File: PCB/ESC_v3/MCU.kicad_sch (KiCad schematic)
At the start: 44 parts, among them J10 Conn_01x01_Pin, J3 Conn_01x01_Pin, J4 Conn_01x01_Pin, J5 Conn_01x01_Pin, J6 Conn_01x01_Pin, J7 Conn_01x01_Pin, J8 Conn_01x01_Pin, J9 Conn_01x01_Pin, U3 STM32G474CETx, Y2 24MHz

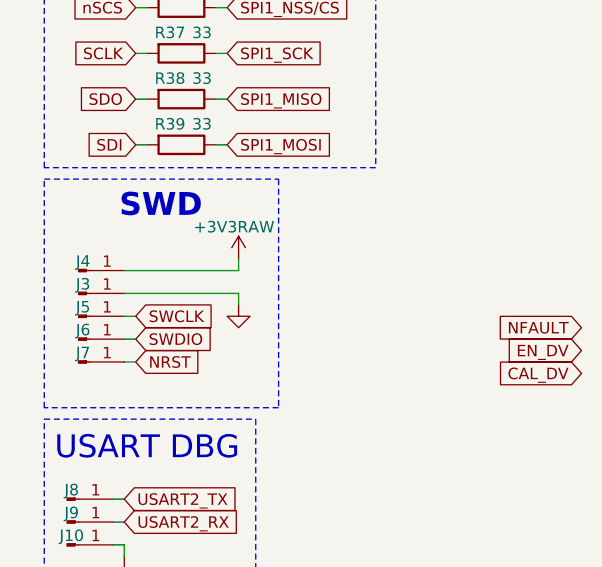
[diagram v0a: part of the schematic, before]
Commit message: Layout update
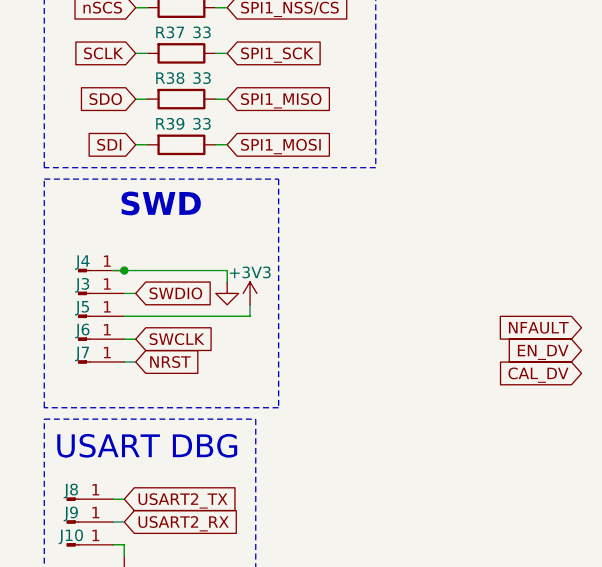
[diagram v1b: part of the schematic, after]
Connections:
- net +3V3RAW is gone; now on net GND: J4.1 (Pin_1)
- net +3V3: now also J5.1 (Pin_1)
- net GND: no longer J3.1 (Pin_1)
- net SWCLK: now also J6.1 (Pin_1); no longer J5.1 (Pin_1)
- net SWDIO: now also J3.1 (Pin_1); no longer J6.1 (Pin_1)
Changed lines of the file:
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@@
 	)
 	(junction
+		(at 25.4 109.22)
+		(diameter 0)
+		(color 0 0 0 0)
+	)
+	(junction
 		(at 43.18 179.07)
 		(diameter 0)
@@
 	(wire
 		(pts
-			(xy 25.4 109.22) (xy 38.1 109.22)
-		)
-		(stroke
-			(width 0)
-			(type default)
-		)
-	)
-	(wire
-		(pts
 			(xy 35.56 60.96) (xy 35.56 62.23)
 		)
@@
 	(wire
 		(pts
-			(xy 25.4 111.76) (xy 38.1 111.76)
-		)
-		(stroke
-			(width 0)
-			(type default)
-		)
-	)
-	(wire
-		(pts
 			(xy 139.7 67.31) (xy 137.16 67.31)
 		)
@@
 	(wire
 		(pts
+			(xy 26.67 111.76) (xy 25.4 111.76)
+		)
+		(stroke
+			(width 0)
+			(type default)
+		)
+	)
+	(wire
+		(pts
 			(xy 25.4 137.16) (xy 24.13 137.16)
 		)
@@
 	(wire
 		(pts
-			(xy 38.1 107.95) (xy 38.1 109.22)
+			(xy 39.37 113.03) (xy 39.37 114.3)
 		)
 		(stroke
@@
 	(wire
 		(pts
-			(xy 38.1 111.76) (xy 38.1 113.03)
+			(xy 36.83 109.22) (xy 36.83 110.49)
 		)
 		(stroke
@@
 	(wire
 		(pts
+			(xy 24.13 109.22) (xy 25.4 109.22)
+		)
+		(stroke
+			(width 0)
+			(type default)
+		)
+	)
+	(wire
+		(pts
 			(xy 43.18 187.96) (xy 43.18 189.23)
 		)
@@
 	(wire
 		(pts
+			(xy 25.4 109.22) (xy 36.83 109.22)
+		)
+		(stroke
+			(width 0)
+			(type default)
+		)
+	)
+	(wire
+		(pts
 			(xy 35.56 85.09) (xy 36.83 85.09)
 		)
@@
 	(wire
 		(pts
-			(xy 26.67 114.3) (xy 25.4 114.3)
+			(xy 25.4 114.3) (xy 39.37 114.3)
 		)
 		(stroke
@@
 	(global_label "SWDIO"
 		(shape input)
-		(at 26.67 116.84 0)
+		(at 26.67 111.76 0)
 		(fields_autoplaced yes)
 		(effects
@@
 		)
 		(property "Intersheetrefs" "${INTERSHEET_REFS}"
-			(at 35.9974 116.84 0)
+			(at 35.9974 111.76 0)
 			(effects
 				(font
@@
 	(global_label "SWCLK"
 		(shape input)
-		(at 26.67 114.3 0)
+		(at 26.67 116.84 0)
 		(fields_autoplaced yes)
 		(effects
@@
 		)
 		(property "Intersheetrefs" "${INTERSHEET_REFS}"
-			(at 36.3602 114.3 0)
+			(at 36.3602 116.84 0)
 			(effects
 				(font
@@
 	)
 	(symbol
+		(lib_id "power:+3V3")
+		(at 39.37 113.03 0)
+		(mirror y)
+		(unit 1)
+		(exclude_from_sim no)
+		(in_bom yes)
+		(on_board yes)
+		(dnp no)
+		(property "Reference" "#PWR035"
+			(at 39.37 116.84 0)
+			(effects
+				(font
+					(size 1.27 1.27)
+				)
+				(hide yes)
+			)
+		)
+		(property "Value" "+3V3"
+			(at 39.37 109.474 0)
+			(effects
+				(font
+					(size 1.27 1.27)
+				)
+			)
+		)
+		(property "Footprint" ""
+			(at 39.37 113.03 0)
+			(effects
+				(font
+					(size 1.27 1.27)
+				)
+				(hide yes)
+			)
+		)
+		(property "Datasheet" ""
+			(at 39.37 113.03 0)
+			(effects
+				(font
+					(size 1.27 1.27)
+				)
+				(hide yes)
+			)
+		)
+		(property "Description" "Power symbol creates a global label with name \"+3V3\""
+			(at 39.37 113.03 0)
+			(effects
+				(font
+					(size 1.27 1.27)
+				)
+				(hide yes)
+			)
+		)
+		(pin "1"
+		)
+		(instances
+			(project "ESC_v3"
+				(path "/bb7f65bd-c3d2-4eba-8e72-fdc4c3d3399c/cb41d658-ae32-4bca-a5d5-9c7fe787c40c"
+					(reference "#PWR035")
+					(unit 1)
+				)
+			)
+		)
+	)
+	(symbol
 		(lib_id "Device:C")
 		(at 39.37 38.1 180)
@@
 	)
 	(symbol
-		(lib_id "power:+3V3")
-		(at 38.1 107.95 0)
-		(unit 1)
-		(exclude_from_sim no)
-		(in_bom yes)
-		(on_board yes)
-		(dnp no)
-		(property "Reference" "#PWR035"
-			(at 38.1 111.76 0)
-			(effects
-				(font
-					(size 1.27 1.27)
-				)
-				(hide yes)
-			)
-		)
-		(property "Value" "+3V3RAW"
-			(at 37.592 104.394 0)
-			(effects
-				(font
-					(size 1.27 1.27)
-				)
-			)
-		)
-		(property "Footprint" ""
-			(at 38.1 107.95 0)
-			(effects
-				(font
-					(size 1.27 1.27)
-				)
-				(hide yes)
-			)
-		)
-		(property "Datasheet" ""
-			(at 38.1 107.95 0)
-			(effects
-				(font
-					(size 1.27 1.27)
-				)
-				(hide yes)
-			)
-		)
-		(property "Description" "Power symbol creates a global label with name \"+3V3\""
-			(at 38.1 107.95 0)
-			(effects
-				(font
-					(size 1.27 1.27)
-				)
-				(hide yes)
-			)
-		)
-		(pin "1"
-		)
-		(instances
-			(project "ESC_v3"
-				(path "/bb7f65bd-c3d2-4eba-8e72-fdc4c3d3399c/cb41d658-ae32-4bca-a5d5-9c7fe787c40c"
-					(reference "#PWR035")
-					(unit 1)
-				)
-			)
-		)
-	)
-	(symbol
 		(lib_id "Device:C")
 		(at 43.18 57.15 180)
@@
 	(symbol
 		(lib_id "power:GND")
-		(at 38.1 113.03 0)
+		(at 36.83 110.49 0)
 		(unit 1)
 		(exclude_from_sim no)
@@
 		(dnp no)
 		(property "Reference" "#PWR030"
-			(at 38.1 119.38 0)
+			(at 36.83 116.84 0)
 			(effects
 				(font
@@
 		)
 		(property "Value" "GND"
-			(at 38.1 116.586 0)
+			(at 36.83 114.046 0)
 			(effects
 				(font
@@
 		)
 		(property "Footprint" ""
-			(at 38.1 113.03 0)
+			(at 36.83 110.49 0)
 			(effects
 				(font
@@
 		)
 		(property "Datasheet" ""
-			(at 38.1 113.03 0)
+			(at 36.83 110.49 0)
 			(effects
 				(font
@@
 		)
 		(property "Description" "Power symbol creates a global label with name \"GND\" , ground"
-			(at 38.1 113.03 0)
+			(at 36.83 110.49 0)
 			(effects
 				(font
